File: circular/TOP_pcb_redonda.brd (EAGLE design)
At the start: 65 x 65 mm, 7 parts

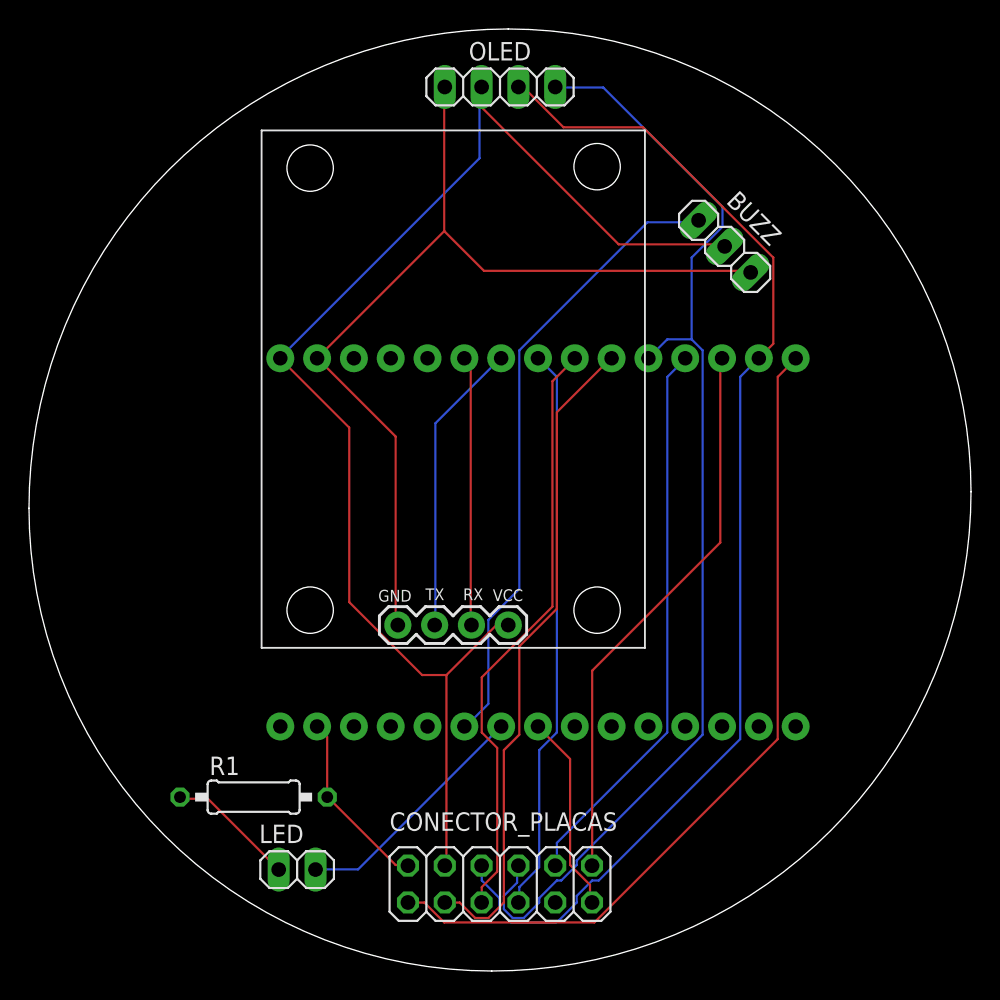
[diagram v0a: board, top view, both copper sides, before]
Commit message: Add files via upload
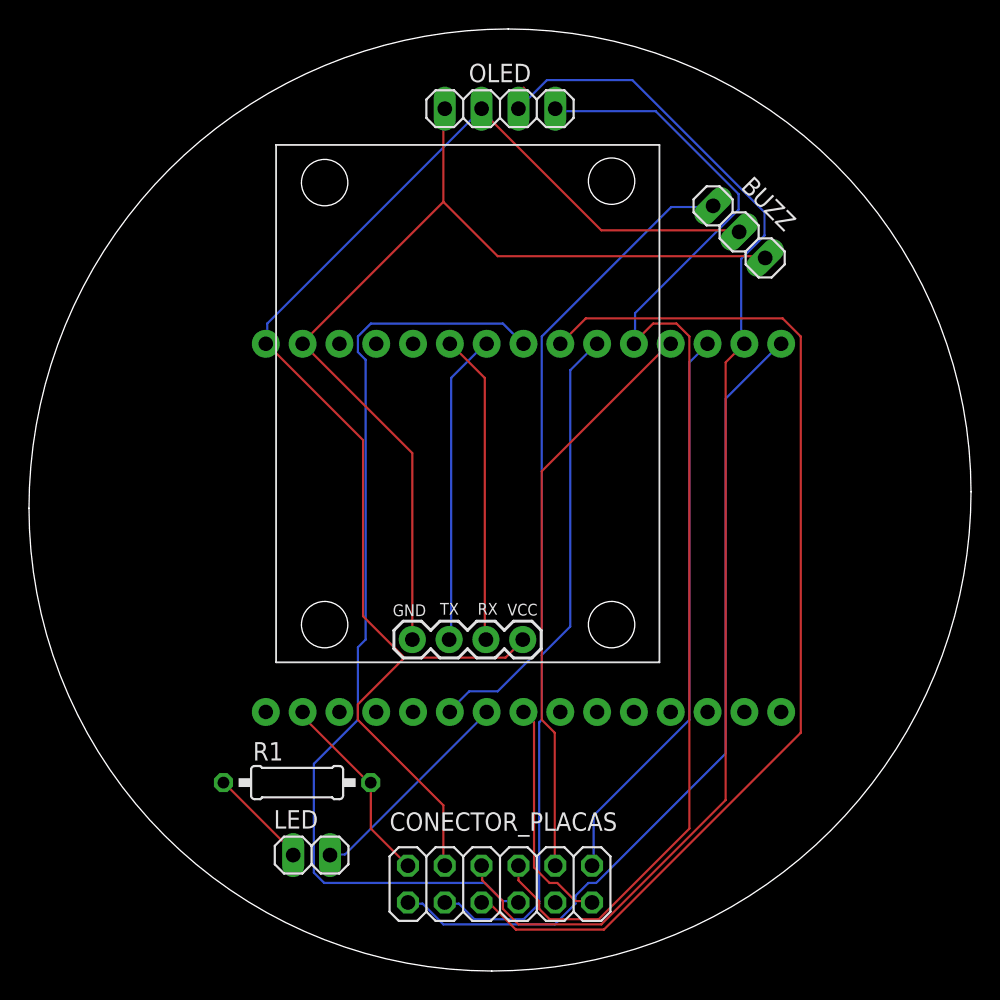
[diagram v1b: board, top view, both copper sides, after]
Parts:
- moved R1 3.16 mm to (18.5, 13.0)
- moved OLED 1.50 mm to (32.5, 59.5)
- moved BUZZ 1.41 mm to (49.0, 51.0)
- moved GPS 1.41 mm to (43.5, 57.0)
- moved LED 1.41 mm to (19.5, 8.00)
- moved PLACA 1.41 mm to (32.9, 31.0)
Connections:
- net N$3 renamed GPS
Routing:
- net N$16: track 41.1 -> 73.6 mm
- net N$17: track 39.2 -> 66.0 mm
- net N$4: track 82.7 -> 88.2 mm
- net N$5: track 79.1 -> 84.0 mm
- net N$1: track 93.1 -> 96.3 mm
- net N$8: track 18.6 -> 21.5 mm
- net N$10: track 13.7 -> 16.0 mm
- net GPS: track 65.5 -> 67.7 mm
- net N$15: track 45.6 -> 47.7 mm
- net N$13: track 43.7 -> 45.5 mm
- net N$11: track 16.9 -> 15.1 mm
- net N$12: track 8.89 -> 7.21 mm
- net N$6: track 38.8 -> 40.1 mm
- net N$9: track 20.3 -> 21.7 mm
- net N$2: track 12.7 -> 13.7 mm
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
